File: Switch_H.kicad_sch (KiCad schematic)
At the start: 11 parts, among them Q201 NVTFWS4D9N04XMTAG, Q202 NVTFWS4D9N04XMTAG, U201 LM74700, U202 LM74700

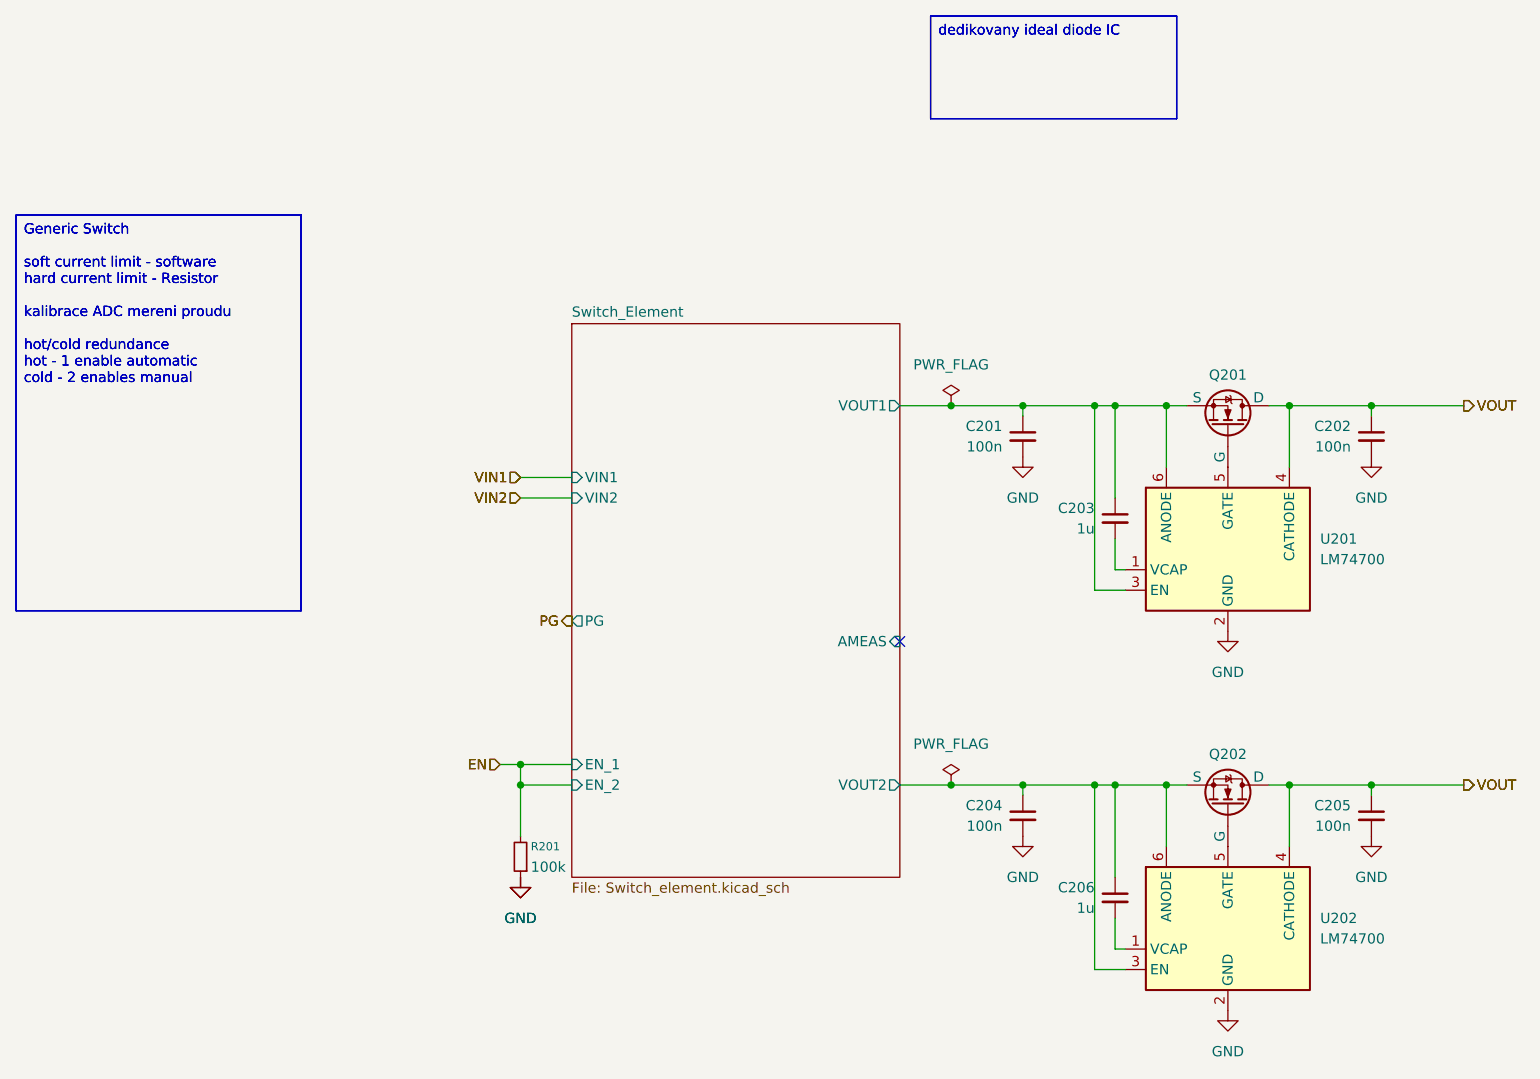
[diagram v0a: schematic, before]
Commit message: small changes to test board
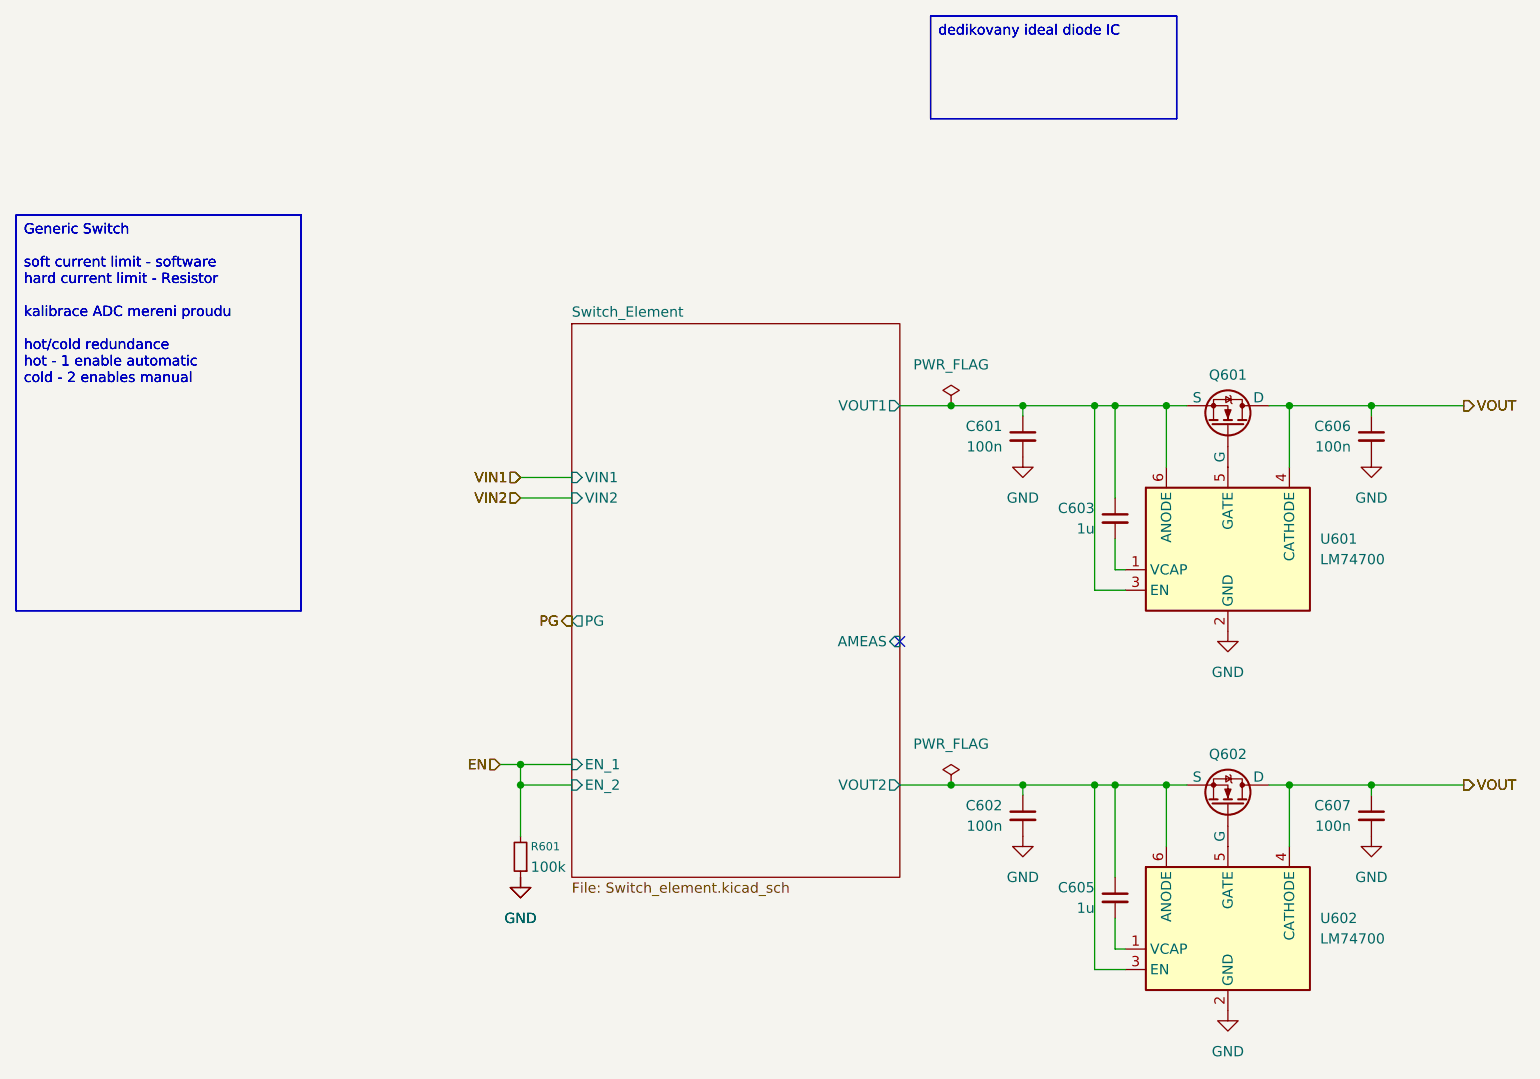
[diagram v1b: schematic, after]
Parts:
- renumbered C201 to C601, C204 to C602, C203 to C603, C206 to C605, C202 to C606, C205 to C607, Q201 to Q601, Q202 to Q602, R201 to R601, U201 to U601, U202 to U602
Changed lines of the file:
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@@
 		(dnp no)
 		(fields_autoplaced yes)
-		(property "Reference" "#PWR0136"
+		(property "Reference" "#PWR0607"
 			(at 191.77 76.2 0)
 			(effects
@@
 		(dnp no)
 		(fields_autoplaced yes)
-		(property "Reference" "#FLG0102"
+		(property "Reference" "#FLG0602"
 			(at 139.7 108.585 0)
 			(effects
@@
 		(dnp no)
 		(fields_autoplaced yes)
-		(property "Reference" "#FLG0101"
+		(property "Reference" "#FLG0601"
 			(at 139.7 61.595 0)
 			(effects
@@
 		(on_board yes)
 		(dnp no)
-		(property "Reference" "R201"
+		(property "Reference" "R601"
 			(at 87.63 118.11 0)
 			(effects
@@
 		(on_board yes)
 		(dnp no)
-		(property "Reference" "Q201"
+		(property "Reference" "Q601"
 			(at 173.99 59.69 90)
 			(effects
@@
 		(dnp no)
 		(fields_autoplaced yes)
-		(property "Reference" "#PWR0131"
+		(property "Reference" "#PWR0601"
 			(at 86.36 128.27 0)
 			(effects
@@
 		(dnp no)
 		(fields_autoplaced yes)
-		(property "Reference" "#PWR0133"
+		(property "Reference" "#PWR0605"
 			(at 173.99 97.79 0)
 			(effects
@@
 		(dnp no)
 		(fields_autoplaced yes)
-		(property "Reference" "#PWR0135"
+		(property "Reference" "#PWR0606"
 			(at 173.99 144.78 0)
 			(effects
@@
 		(dnp no)
 		(fields_autoplaced yes)
-		(property "Reference" "#PWR0137"
+		(property "Reference" "#PWR0603"
 			(at 148.59 76.2 0)
 			(effects
@@
 		(dnp no)
 		(fields_autoplaced yes)
-		(property "Reference" "#PWR0134"
+		(property "Reference" "#PWR0608"
 			(at 191.77 123.19 0)
 			(effects
@@
 		(dnp no)
 		(fields_autoplaced yes)
-		(property "Reference" "U202"
+		(property "Reference" "U602"
 			(at 185.42 126.9999 0)
 			(effects
@@
 		(on_board yes)
 		(dnp no)
-		(property "Reference" "C204"
+		(property "Reference" "C602"
 			(at 146.05 113.0362 0)
 			(effects
@@
 		(on_board yes)
 		(dnp no)
-		(property "Reference" "C203"
+		(property "Reference" "C603"
 			(at 157.48 76.2062 0)
 			(effects
@@
 		(on_board yes)
 		(dnp no)
-		(property "Reference" "C201"
+		(property "Reference" "C601"
 			(at 146.05 66.0462 0)
 			(effects
@@
 		(on_board yes)
 		(dnp no)
-		(property "Reference" "C202"
+		(property "Reference" "C606"
 			(at 189.23 66.0462 0)
 			(effects
@@
 		(dnp no)
 		(fields_autoplaced yes)
-		(property "Reference" "#PWR0138"
+		(property "Reference" "#PWR0604"
 			(at 148.59 123.19 0)
 			(effects
@@
 		(on_board yes)
 		(dnp no)
-		(property "Reference" "C205"
+		(property "Reference" "C607"
 			(at 189.23 113.0362 0)
 			(effects
@@
 		(on_board yes)
 		(dnp no)
-		(property "Reference" "Q202"
+		(property "Reference" "Q602"
 			(at 173.99 106.68 90)
 			(effects
@@
 		(dnp no)
 		(fields_autoplaced yes)
-		(property "Reference" "U201"
+		(property "Reference" "U601"
 			(at 185.42 80.0099 0)
 			(effects
@@
 		(dnp no)
 		(fields_autoplaced yes)
-		(property "Reference" "#PWR0132"
+		(property "Reference" "#PWR0602"
 			(at 86.36 128.27 0)
 			(effects
@@
 		(on_board yes)
 		(dnp no)
-		(property "Reference" "C206"
+		(property "Reference" "C605"
 			(at 157.48 123.1962 0)
 			(effects

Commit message: nearly finnished CORE pcb
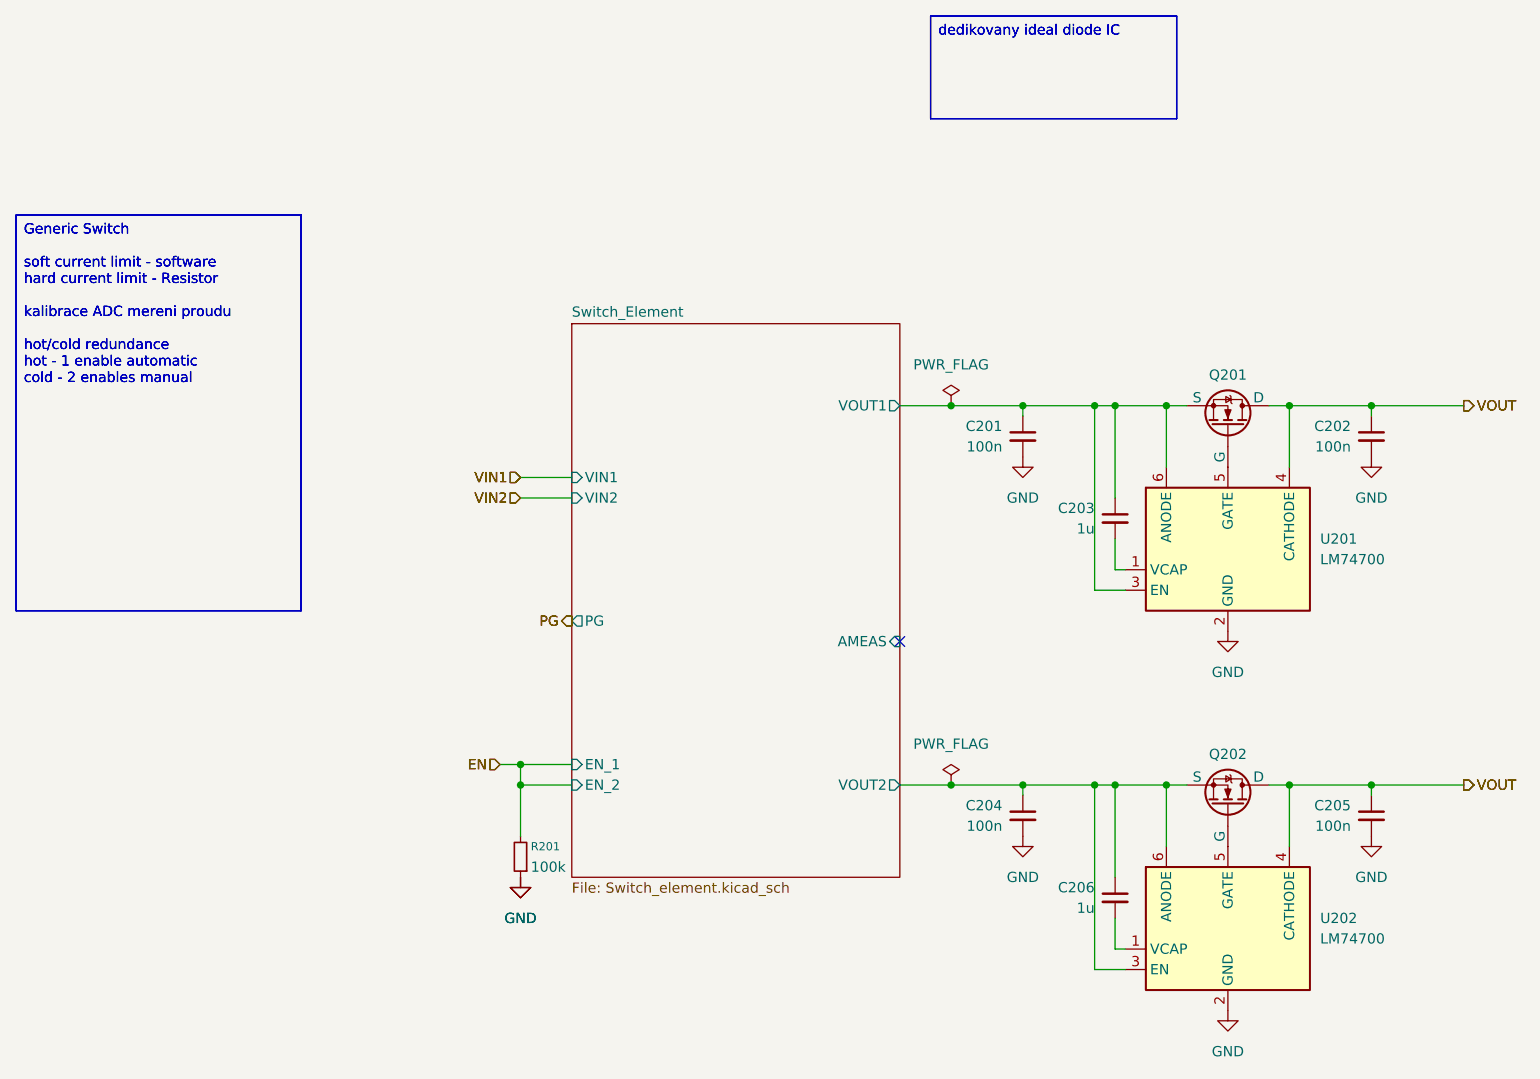
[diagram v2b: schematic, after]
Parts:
- renumbered C601 to C201, C606 to C202, C603 to C203, C602 to C204, C607 to C205, C605 to C206, Q601 to Q201, Q602 to Q202, R601 to R201, U601 to U201, U602 to U202
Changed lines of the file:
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@@
 		(dnp no)
 		(fields_autoplaced yes)
-		(property "Reference" "#PWR0607"
+		(property "Reference" "#PWR0136"
 			(at 191.77 76.2 0)
 			(effects
@@
 		(dnp no)
 		(fields_autoplaced yes)
-		(property "Reference" "#FLG0602"
+		(property "Reference" "#FLG0102"
 			(at 139.7 108.585 0)
 			(effects
@@
 		(dnp no)
 		(fields_autoplaced yes)
-		(property "Reference" "#FLG0601"
+		(property "Reference" "#FLG0101"
 			(at 139.7 61.595 0)
 			(effects
@@
 		(on_board yes)
 		(dnp no)
-		(property "Reference" "R601"
+		(property "Reference" "R201"
 			(at 87.63 118.11 0)
 			(effects
@@
 		(on_board yes)
 		(dnp no)
-		(property "Reference" "Q601"
+		(property "Reference" "Q201"
 			(at 173.99 59.69 90)
 			(effects
@@
 		(dnp no)
 		(fields_autoplaced yes)
-		(property "Reference" "#PWR0601"
+		(property "Reference" "#PWR0131"
 			(at 86.36 128.27 0)
 			(effects
@@
 		(dnp no)
 		(fields_autoplaced yes)
-		(property "Reference" "#PWR0605"
+		(property "Reference" "#PWR0133"
 			(at 173.99 97.79 0)
 			(effects
@@
 		(dnp no)
 		(fields_autoplaced yes)
-		(property "Reference" "#PWR0606"
+		(property "Reference" "#PWR0135"
 			(at 173.99 144.78 0)
 			(effects
@@
 		(dnp no)
 		(fields_autoplaced yes)
-		(property "Reference" "#PWR0603"
+		(property "Reference" "#PWR0137"
 			(at 148.59 76.2 0)
 			(effects
@@
 		(dnp no)
 		(fields_autoplaced yes)
-		(property "Reference" "#PWR0608"
+		(property "Reference" "#PWR0134"
 			(at 191.77 123.19 0)
 			(effects
@@
 		(dnp no)
 		(fields_autoplaced yes)
-		(property "Reference" "U602"
+		(property "Reference" "U202"
 			(at 185.42 126.9999 0)
 			(effects
@@
 		(on_board yes)
 		(dnp no)
-		(property "Reference" "C602"
+		(property "Reference" "C204"
 			(at 146.05 113.0362 0)
 			(effects
@@
 		(on_board yes)
 		(dnp no)
-		(property "Reference" "C603"
+		(property "Reference" "C203"
 			(at 157.48 76.2062 0)
 			(effects
@@
 		(on_board yes)
 		(dnp no)
-		(property "Reference" "C601"
+		(property "Reference" "C201"
 			(at 146.05 66.0462 0)
 			(effects
@@
 		(on_board yes)
 		(dnp no)
-		(property "Reference" "C606"
+		(property "Reference" "C202"
 			(at 189.23 66.0462 0)
 			(effects
@@
 		(dnp no)
 		(fields_autoplaced yes)
-		(property "Reference" "#PWR0604"
+		(property "Reference" "#PWR0138"
 			(at 148.59 123.19 0)
 			(effects
@@
 		(on_board yes)
 		(dnp no)
-		(property "Reference" "C607"
+		(property "Reference" "C205"
 			(at 189.23 113.0362 0)
 			(effects
@@
 		(on_board yes)
 		(dnp no)
-		(property "Reference" "Q602"
+		(property "Reference" "Q202"
 			(at 173.99 106.68 90)
 			(effects
@@
 		(dnp no)
 		(fields_autoplaced yes)
-		(property "Reference" "U601"
+		(property "Reference" "U201"
 			(at 185.42 80.0099 0)
 			(effects
@@
 		(dnp no)
 		(fields_autoplaced yes)
-		(property "Reference" "#PWR0602"
+		(property "Reference" "#PWR0132"
 			(at 86.36 128.27 0)
 			(effects
@@
 		(on_board yes)
 		(dnp no)
-		(property "Reference" "C605"
+		(property "Reference" "C206"
 			(at 157.48 123.1962 0)
 			(effects
